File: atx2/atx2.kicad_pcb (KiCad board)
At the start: 2 copper layers, 33.7 x 85.6 mm, 6 parts, among them J1 ATX-24, J2 Conn_02x02_Top_Bottom, J3 Conn_01x02, J4 Conn_01x02, J5 Conn_01x02, J6 Conn_02x02_Top_Bottom

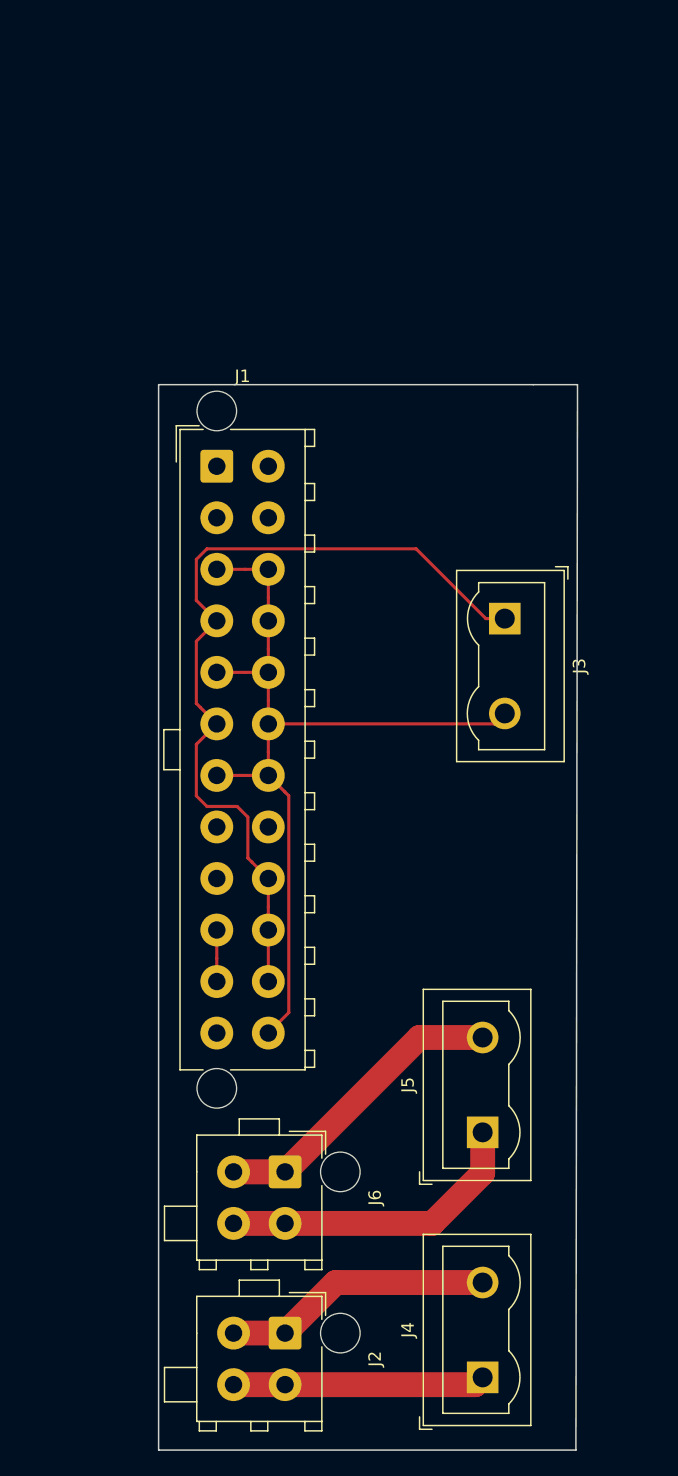
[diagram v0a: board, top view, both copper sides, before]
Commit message: design-v1
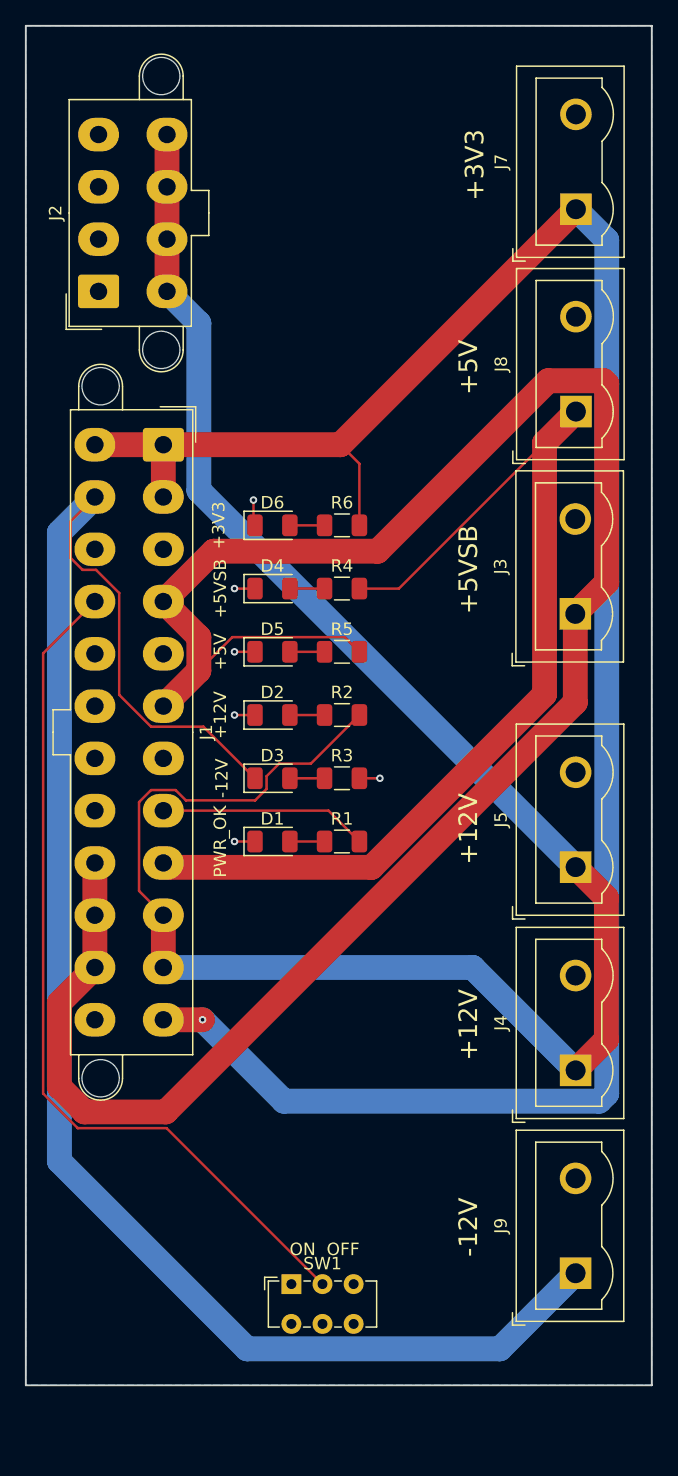
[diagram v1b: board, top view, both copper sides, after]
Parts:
- removed J6: Conn_02x02_Top_Bottom, Connector_TE-Connectivity:TE_MATE-N-LOK_1-770874-x_2x02_P4.14mm_Vertical
- added D1: LED, LED_SMD:LED_1206_3216Metric, F.Cu at (72.6, 107.7)
- added D2: LED, LED_SMD:LED_1206_3216Metric, F.Cu at (72.6, 97.5)
- added D3: LED, LED_SMD:LED_1206_3216Metric, F.Cu at (72.6, 102.6)
- added D4: LED, LED_SMD:LED_1206_3216Metric, F.Cu at (72.6, 87.4)
- added D5: LED, LED_SMD:LED_1206_3216Metric, F.Cu at (72.6, 92.5)
- added D6: LED, LED_SMD:LED_1206_3216Metric, F.Cu at (72.6, 82.3)
- added J7: Conn_01x02, TerminalBlock:TerminalBlock_Wuerth_691311400102_P7.62mm, F.Cu at (97.0, 56.9)
- added J8: Conn_01x02, TerminalBlock:TerminalBlock_Wuerth_691311400102_P7.62mm, F.Cu at (97.0, 73.2)
- added J9: Conn_01x02, TerminalBlock:TerminalBlock_Wuerth_691311400102_P7.62mm, F.Cu at (97.0, 142.4)
- added R1: 220, Resistor_SMD:R_1206_3216Metric, F.Cu at (78.2, 107.7)
- added R2: 510, Resistor_SMD:R_1206_3216Metric, F.Cu at (78.2, 97.5)
- added R3: 510, Resistor_SMD:R_1206_3216Metric, F.Cu at (78.2, 102.6)
- added R4: 220, Resistor_SMD:R_1206_3216Metric, F.Cu at (78.2, 87.4)
- added R5: 220, Resistor_SMD:R_1206_3216Metric, F.Cu at (78.2, 92.5)
- added R6: 68, Resistor_SMD:R_1206_3216Metric, F.Cu at (78.2, 82.3)
- added SW1: SW_SPDT, Button_Switch_THT:SW_E-Switch_EG1271_DPDT, F.Cu at (74.2, 143.3)
- J1: footprint Connector_TE-Connectivity:TE_MATE-N-LOK_1-794072-x_2x12_P4.14mm_Vertical -> Connector_Molex:Molex_Mini-Fit_Jr_5566-24A2_2x12_P4.20mm_Vertical
- J2: value Conn_02x02_Top_Bottom -> Conn_02x04_Top_Bottom; footprint Connector_TE-Connectivity:TE_MATE-N-LOK_1-770874-x_2x02_P4.14mm_Vertical -> Connector_Molex:Molex_Mini-Fit_Jr_5566-08A2_2x04_P4.20mm_Vertical
- moved J2 85.0 mm to (58.7, 63.5), turned to 90 degrees
- moved J4 25.8 mm to (97.0, 126.1)
- moved J5 22.6 mm to (97.0, 109.8)
- moved J3 5.68 mm to (97.0, 89.4), turned to 90 degrees
- moved J1 4.63 mm to (63.9, 75.8), turned to 270 degrees
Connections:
- net Net-(J1-Pad1) renamed +3V3
- J1 pad 14: Net-(J1-Pad14) -> -12V
- J1 pad 16: GND -> Net-(J1-Pad16)
- J1 pad 9: Net-(J1-Pad9) -> +5VA
- J2 pad 3: +12V -> GND
- J2 pad 4: +12V -> GND
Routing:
- net +3V3: track 0.00 -> 168.5 mm, vias 0 -> 1
- net -12V: track 0.00 -> 137.4 mm
- net +12V: track 49.4 -> 163.4 mm
- net GND: track 116.6 -> 10.3 mm, vias 0 -> 6
- net +5V: track 67.9 -> 174.1 mm
- net +5VA: track 0.00 -> 83.6 mm
- net Net-(J1-Pad16): track 0.00 -> 70.0 mm
- net Net-(J1-Pad8): track 0.00 -> 16.8 mm
- net Net-(D6-Pad2): track 0.00 -> 2.79 mm
- net Net-(D5-Pad2): track 0.00 -> 2.79 mm
- net Net-(D4-Pad2): track 0.00 -> 2.79 mm
- net Net-(D3-Pad2): track 0.00 -> 2.79 mm
- net Net-(D2-Pad2): track 0.00 -> 2.79 mm
- net Net-(D1-Pad2): track 0.00 -> 2.79 mm
- added copper zone on B.Cu, net GND
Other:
- board size 33.7 x 85.6 mm -> 50.3 x 109.2 mm
- net class Default: clearance 0.2 -> 0.2032; trace_width 0.25 -> 0.2032; via_dia 0.8 -> 0.6; via_drill 0.4 -> 0.3
- rule trace_clearance: 0.2 -> 0.2032
- rule trace_min: 0.2 -> 0.2032
- board text added: "+12V"
- board text added: "+3V3"
- board text added: "+5V"
- board text added: "+5VSB"
- board text added: "-12V"
- board text added: "ON OFF"
- board text added: "PWR_OK"
